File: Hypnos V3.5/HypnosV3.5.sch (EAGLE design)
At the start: 39 parts, among them J1 MEM2051-00-195-00-A_REVD1MEM2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, Q1 DMN65D8L-7, Q2 DMN65D8L-7

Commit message: Add files via upload
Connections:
- net GND: now also MICROSD.CARD_DETECT1
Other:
- moved on the sheet: +IN, 3V, 3V|5V, 5V, BT1, C1, C2, C3, CS, D1, D2, INT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

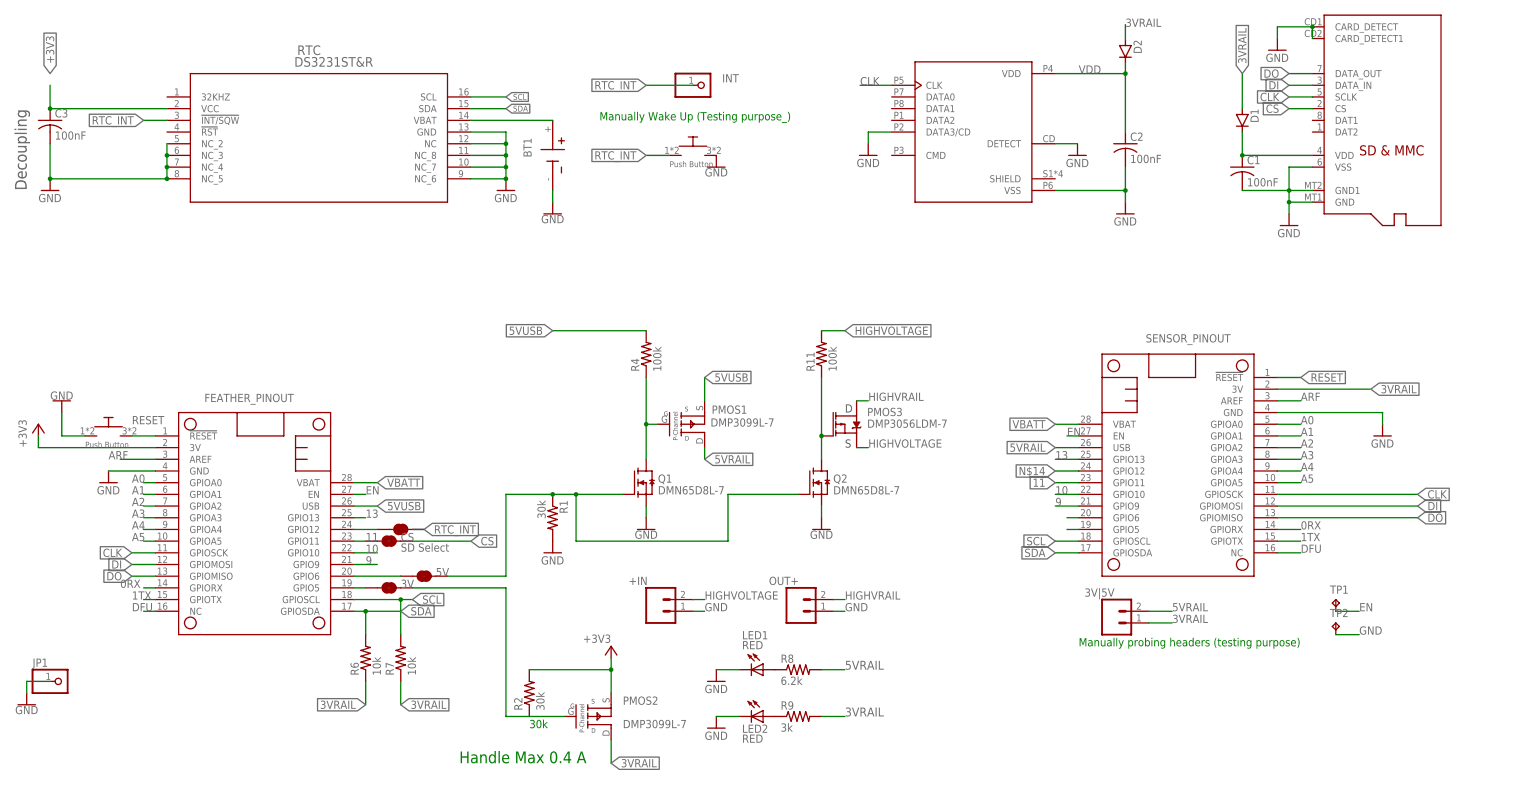
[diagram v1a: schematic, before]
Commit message: Add files via upload
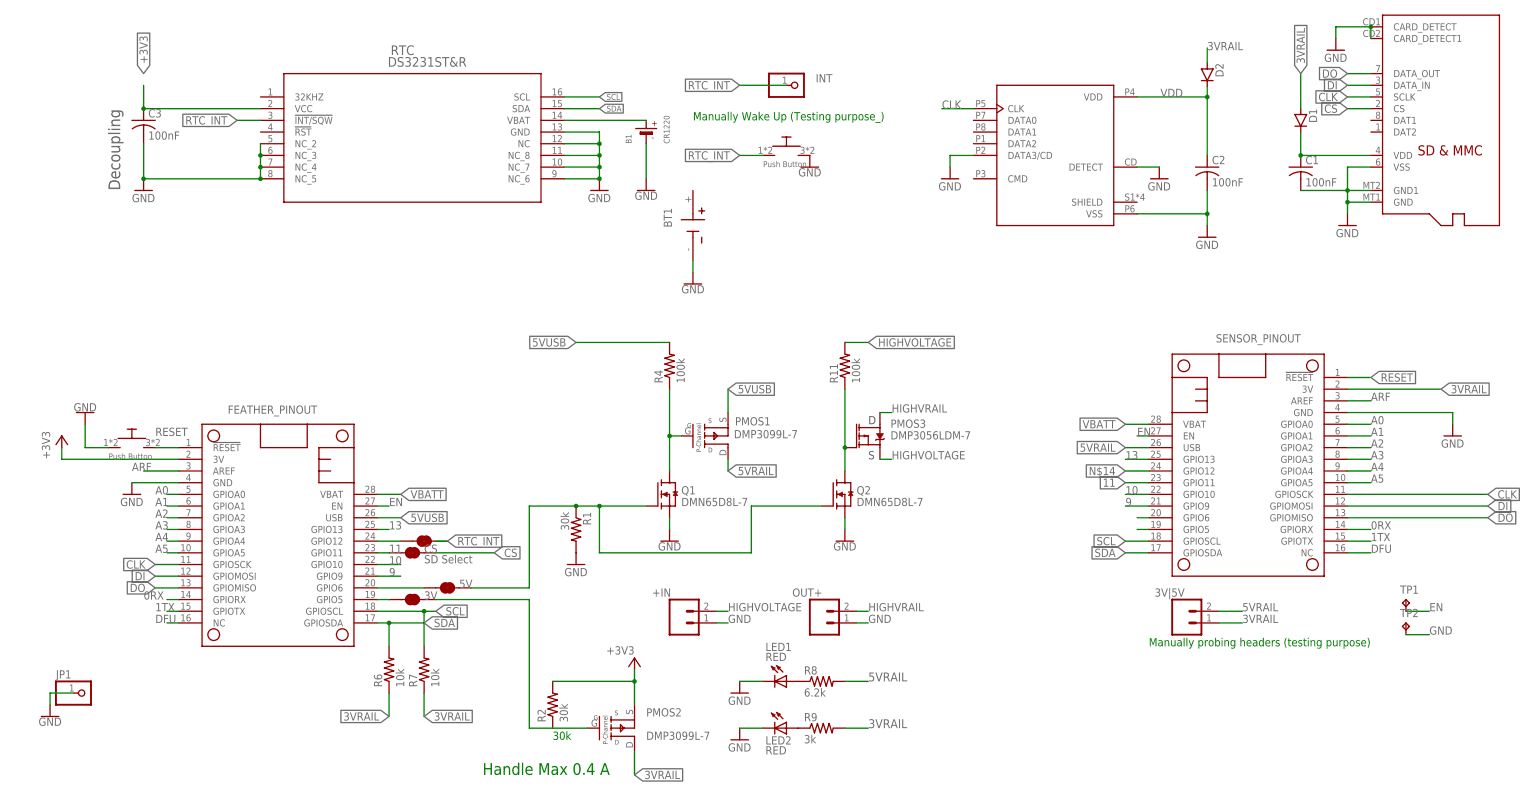
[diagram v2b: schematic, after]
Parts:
- added B1: CR1220, microbuilder:BATTERYCR1220_SMT
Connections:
- net GND: now also B1.-
- net N$2: now also B1.+; no longer BT1.+
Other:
- moved on the sheet: +IN, 3V, 3V|5V, 5V, BT1, C1, C2, C3, CS, D1, D2, INT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

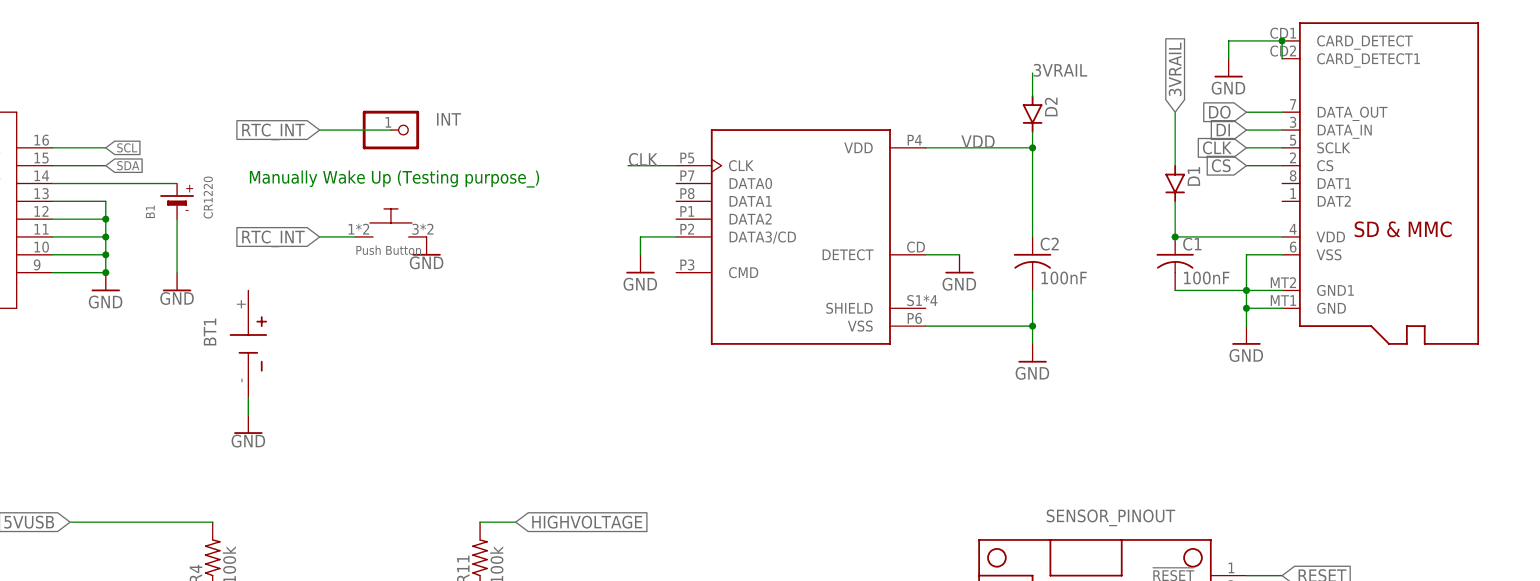
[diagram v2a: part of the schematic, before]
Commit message: Add files via upload
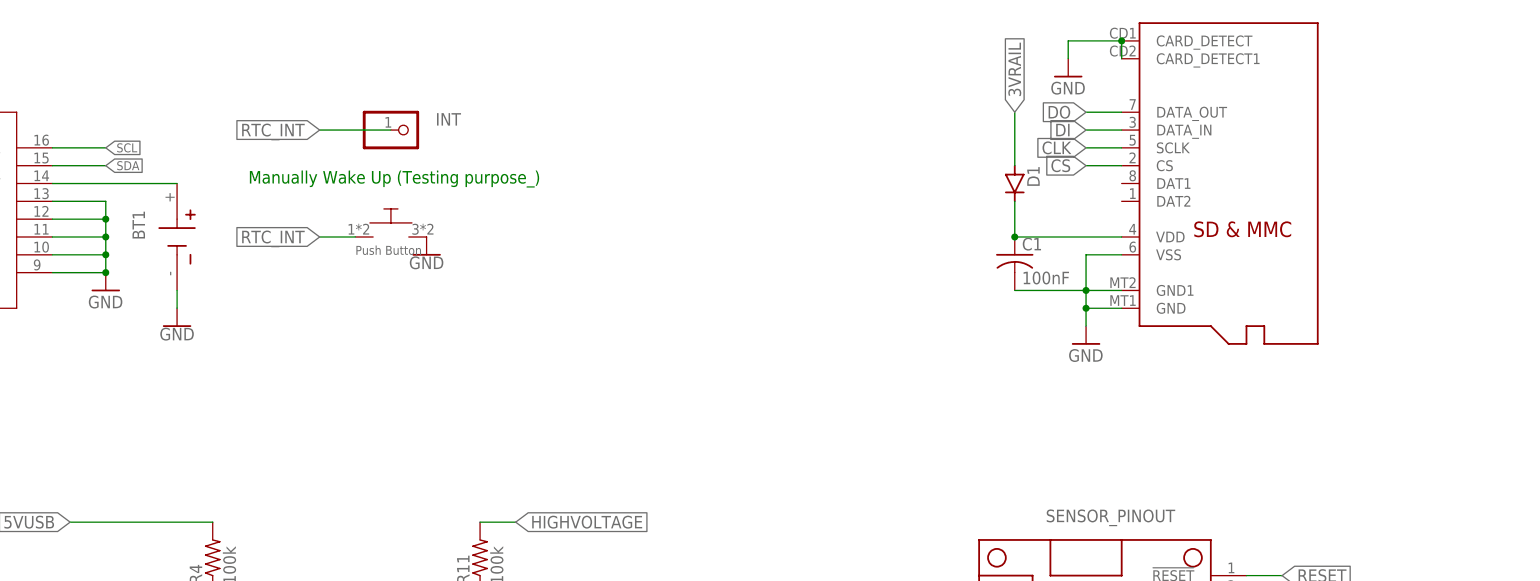
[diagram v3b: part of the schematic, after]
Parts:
- removed B1: CR1220, microbuilder:BATTERYCR1220_SMT
- removed C2: 100nF, adafruit:C-USC1206
- removed D2: (no value), semicon-smd-ipc:D-SOD123
- removed J1: MEM2051-00-195-00-A_REVD1MEM2051-00-195-00-A_GCT_MEM2051-00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, MEM2051-00-195-00-A_REVD1:MEM2051-00-195-00-A_REVD1MEM2051-00-195-00-A_GCT_MEM2051-00-195-00-A
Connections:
- net 3VRAIL: no longer D2.A
- net CLK: no longer J1.CLK
- net GND: no longer B1.-, C2.2, J1.DATA3/CD, J1.DETECT, J1.VSS
- net N$2: now also BT1.+; no longer B1.+
- net VDD: no longer C2.1, D2.C, J1.VDD
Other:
- moved on the sheet: BT1, C1, D1
